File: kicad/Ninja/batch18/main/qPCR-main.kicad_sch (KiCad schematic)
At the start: 24 parts, among them J1 Barrel_Jack_Switch, J19 Conn_01x08_Male, J2 Raspberry_Pi_3A_Plus_wpi, J5 Conn_01x10_Male, Q1 Q_NMOS_GSD, Q2 Q_NMOS_GSD, Q3 Q_NMOS_GSD, Q5 Q_NMOS_GSD, SW1 SW_Reed, U5 DIN4_PWR

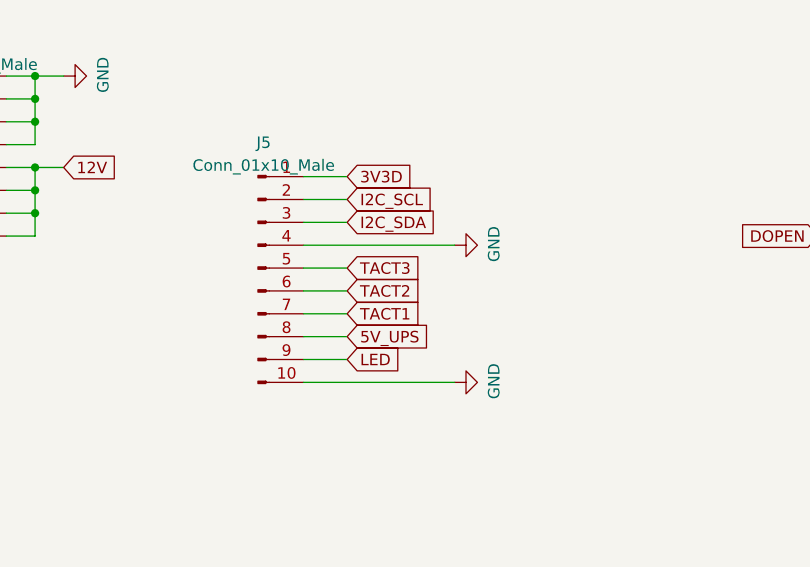
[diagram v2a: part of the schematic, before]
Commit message: wired batch03/main
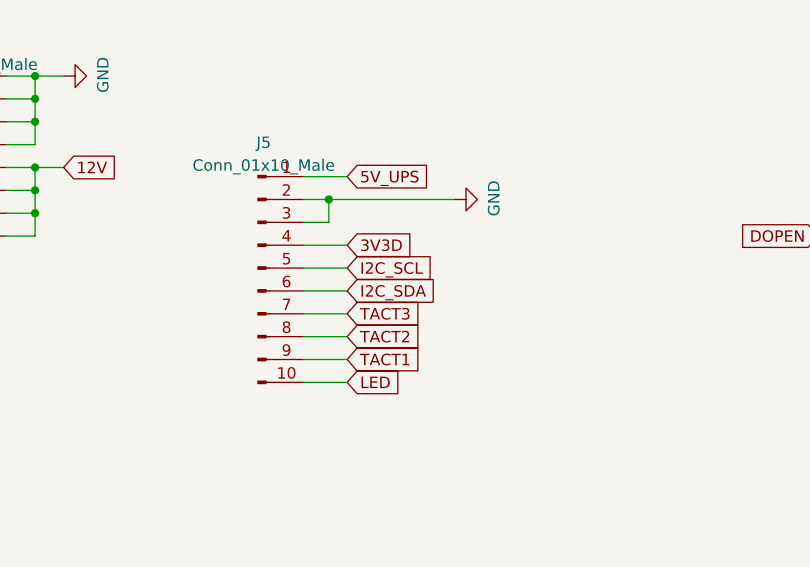
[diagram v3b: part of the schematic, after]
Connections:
- net 3V3D: now also J5.4 (Pin_4); no longer J5.1 (Pin_1)
- net 5V_UPS: now also J5.1 (Pin_1); no longer J5.8 (Pin_8)
- net GND: now also J5.2 (Pin_2), J5.3 (Pin_3); no longer J5.10 (Pin_10), J5.4 (Pin_4)
- net I2C_SCL: now also J5.5 (Pin_5); no longer J5.2 (Pin_2)
- net I2C_SDA: now also J5.6 (Pin_6); no longer J5.3 (Pin_3)
- net LED: now also J5.10 (Pin_10); no longer J5.9 (Pin_9)
- net TACT1: now also J5.9 (Pin_9); no longer J5.7 (Pin_7)
- net TACT2: now also J5.8 (Pin_8); no longer J5.6 (Pin_6)
- net TACT3: now also J5.7 (Pin_7); no longer J5.5 (Pin_5)
